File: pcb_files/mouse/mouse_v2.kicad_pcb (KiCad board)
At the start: 2 copper layers, 94.7 x 94.9 mm, 51 parts, among them J2 BT_Conn, J4 I2C_Conn, M1 Motor_DC, M2 Motor_DC, M3 CASTER_BALL, Q0 Q_Photo_NPN, Q1 Q_Photo_NPN, Q2 Q_Photo_NPN, Q3 Q_Photo_NPN, SW1 SW_Push, T0 Q_NMOS_DGS, T1 Q_NMOS_DGS, T2 Q_NMOS_DGS, T3 Q_NMOS_DGS, U1 Teensy3.2, U2 SN754410NE, U3 LM1084-5.0, U4 Encoder_3081, U5 Encoder_3081

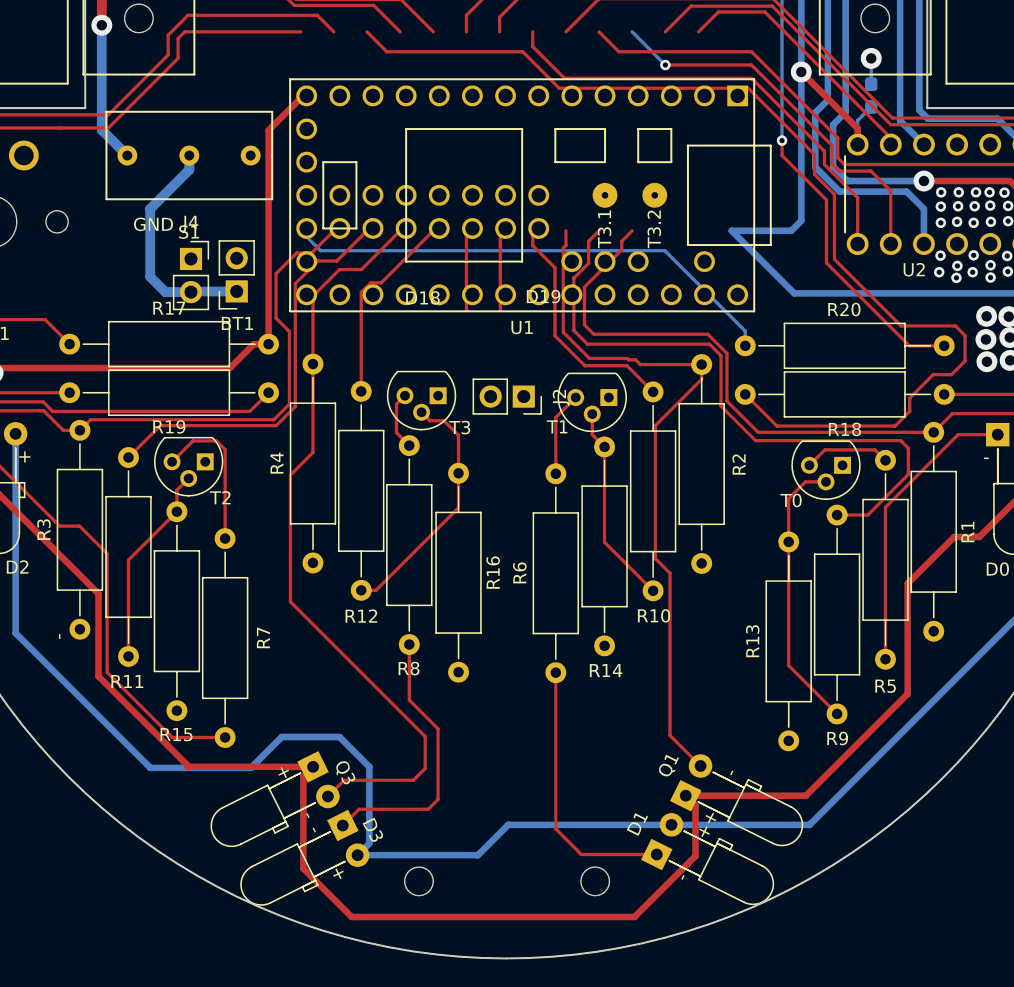
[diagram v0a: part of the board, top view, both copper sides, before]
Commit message: added rgb led to schematic
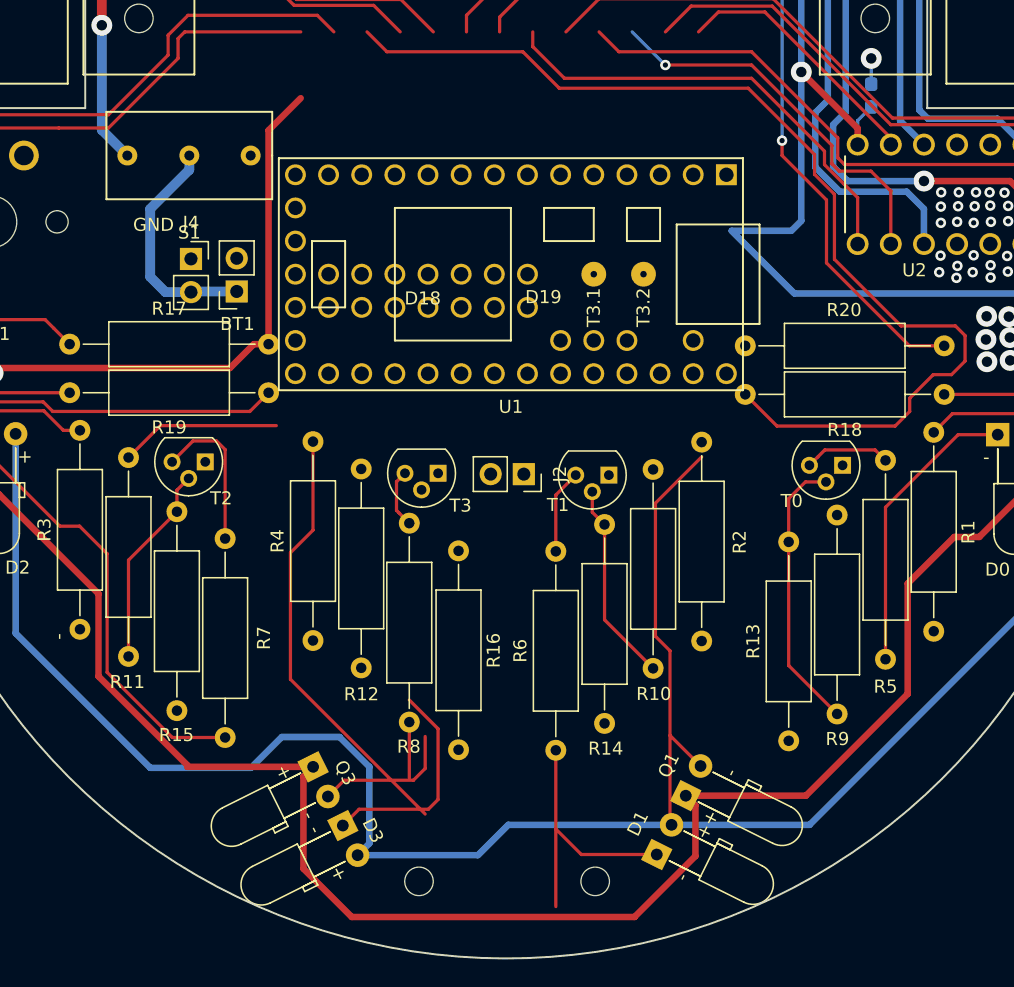
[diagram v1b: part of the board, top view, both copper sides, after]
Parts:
- moved U1 6.11 mm to (158.9, 97.3)
- moved R8 5.94 mm to (151.1, 131.6)
- moved R14 5.94 mm to (166.0, 131.7)
- moved R6 5.94 mm to (162.3, 133.8)
- moved T3 5.94 mm to (153.3, 112.6)
- moved J2 5.94 mm to (159.8, 112.6)
- moved R10 5.94 mm to (169.7, 127.5)
- moved R12 5.94 mm to (147.4, 127.5)
- moved R16 5.94 mm to (154.8, 133.7)
- moved R2 5.94 mm to (173.5, 125.4)
- moved R4 5.94 mm to (143.7, 125.4)
- moved T1 5.94 mm to (166.4, 112.7)
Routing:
- net /Emitter_0: track 48.8 -> 0.00 mm
- net /Reciever_0: track 55.5 -> 14.5 mm
- net /Buzzer: track 38.4 -> 0.00 mm
- net /Reciever_2: track 45.5 -> 12.4 mm
- net /Reciever_1: track 53.1 -> 32.5 mm
- net Net-(R12-Pad1): track 19.2 -> 0.00 mm
- net /Emitter_2: track 31.0 -> 12.3 mm
- net /Emitter_1: track 18.1 -> 0.00 mm
- net /Emitter_3: track 15.1 -> 0.00 mm
- net /Reciever_3: track 58.3 -> 44.3 mm
- net Net-(U1-Pad50): track 6.10 -> 0.00 mm
- net Net-(U1-Pad49): track 6.14 -> 0.07 mm
